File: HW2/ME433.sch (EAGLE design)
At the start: 22 parts, among them J1 USB-MB-H

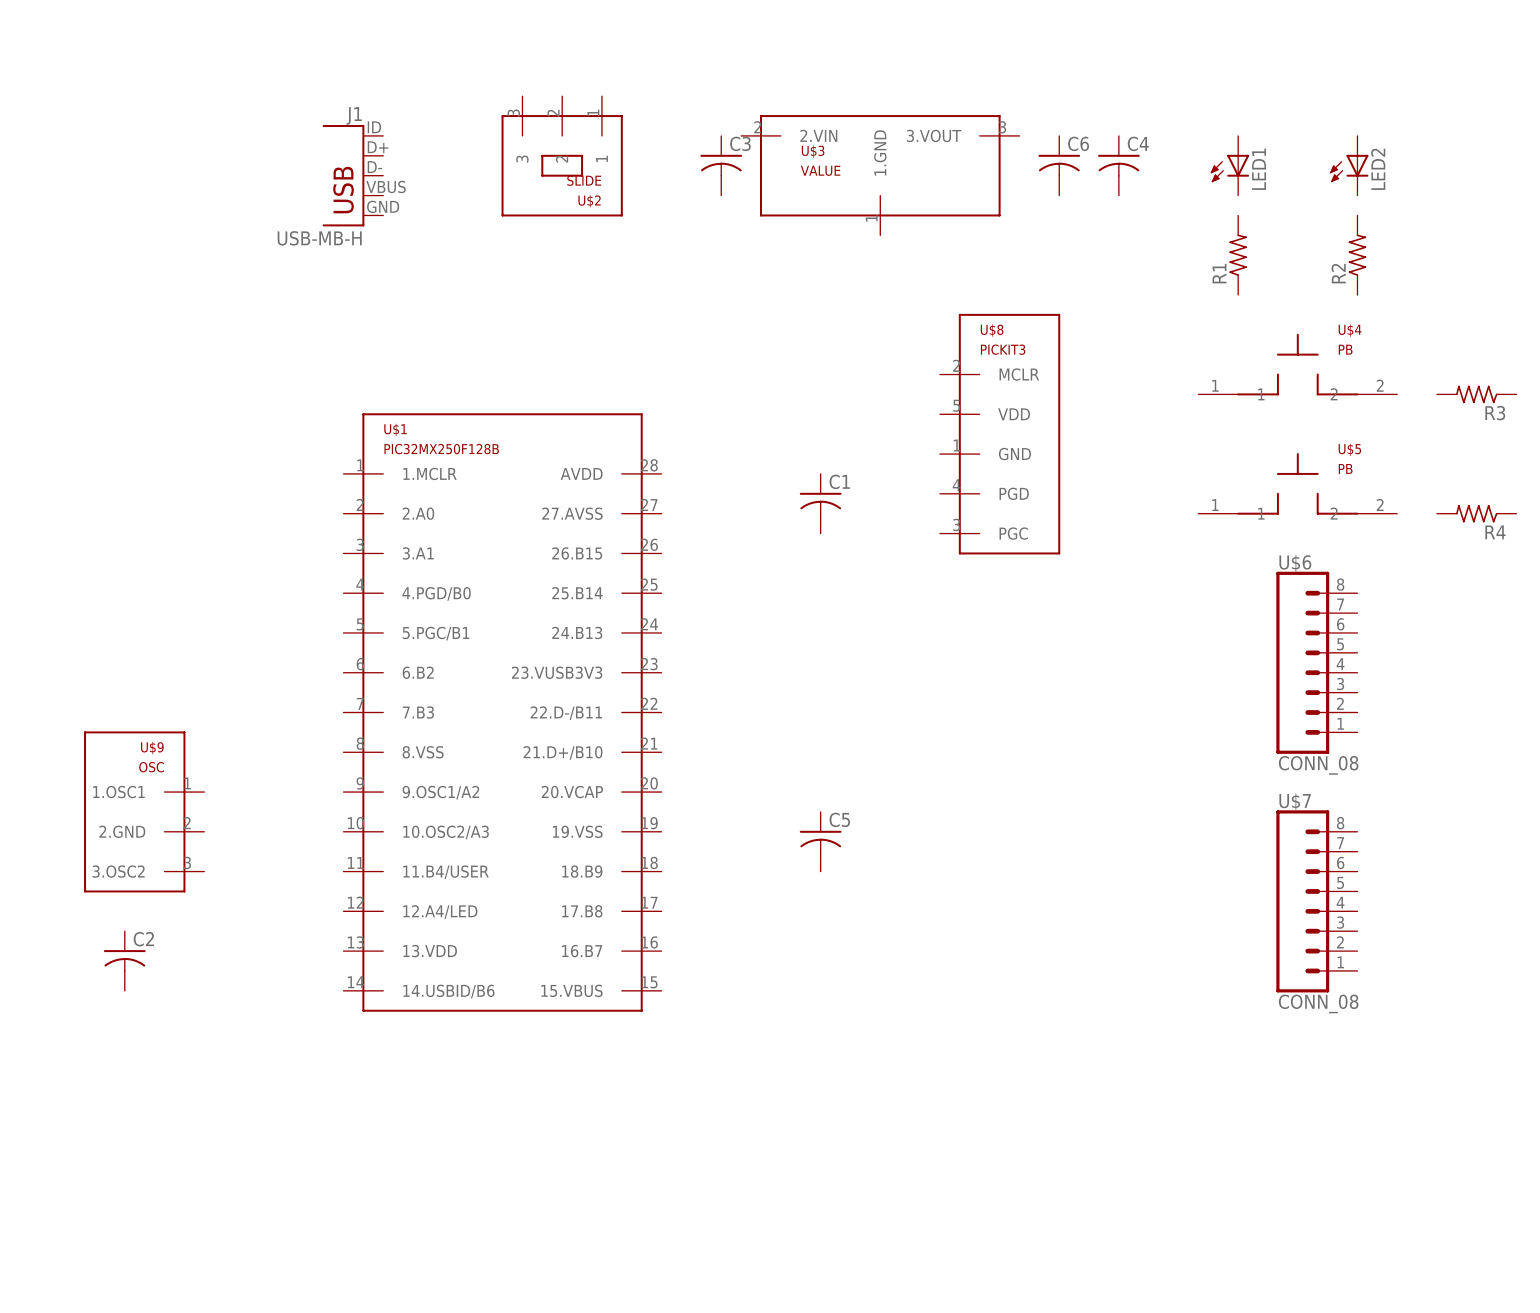
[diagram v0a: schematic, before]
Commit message: cleaned up HW2
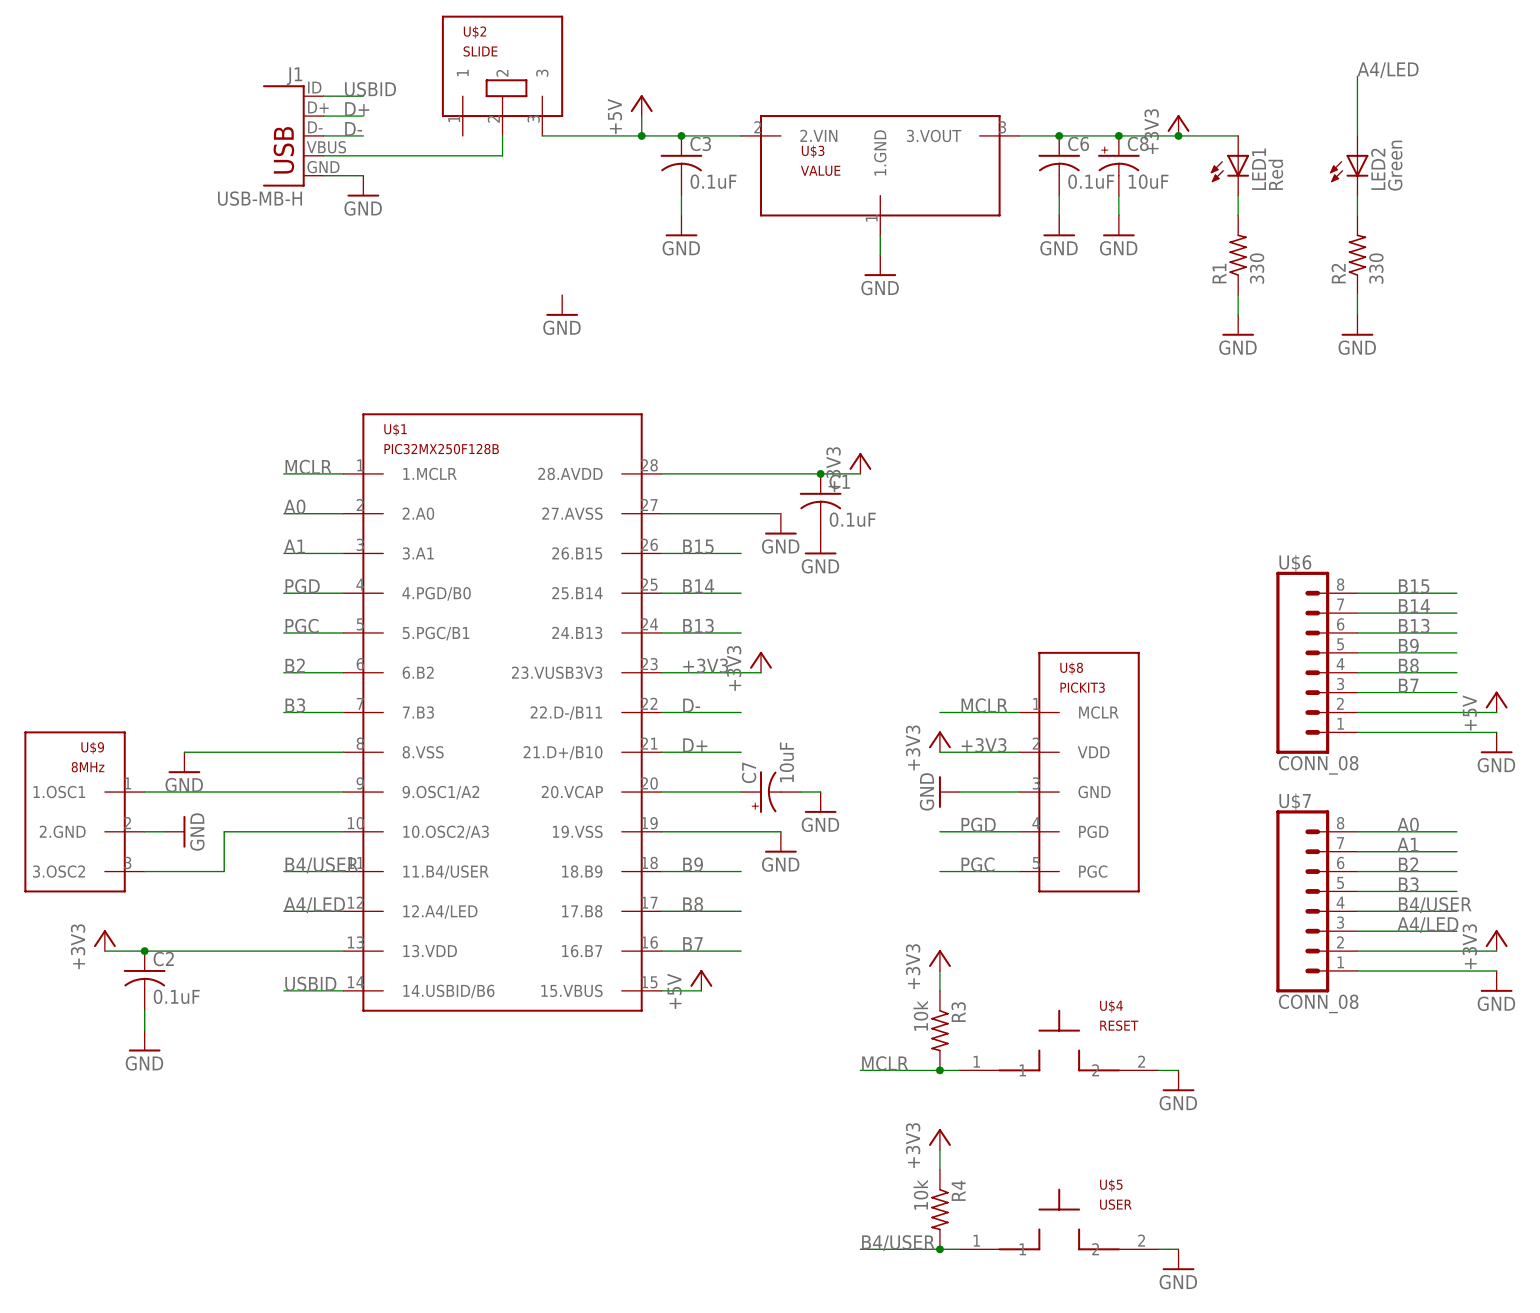
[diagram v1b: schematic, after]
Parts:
- removed C4, C5: (no value), resistor:C-US025-025X050
- added C7, C8: 10uF, HW2:CPOL-USB45181B
- C1, C2, C3, C6: value (none) -> 0.1uF
- LED1: value (none) -> Red
- LED2: value (none) -> Green
- R1, R2: value (none) -> 330
- R3, R4: value (none) -> 10k
- U$4: value PB -> RESET
- U$5: value PB -> USER
- U$9: value OSC -> 8MHz
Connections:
- new net +3V3: C1.1, C2.1, C6.1, C8.+, LED1.A, R3.1, R4.1, U$1.13.VDD, U$1.23.VUSB3V3, U$1.28.AVDD, U$3.3.VOUT, U$7.2, U$8.VDD
- new net +5V: C3.1, U$1.15.VBUS, U$2.3, U$3.2.VIN, U$6.2
- new net A0: U$1.2.A0, U$7.8
- new net A1: U$1.3.A1, U$7.7
- new net A4/LED: LED2.A, U$1.12.A4/LED, U$7.3
- new net B13: U$1.24.B13, U$6.6
- new net B14: U$1.25.B14, U$6.7
- new net B15: U$1.26.B15, U$6.8
- new net B2: U$1.6.B2, U$7.6
- new net B3: U$1.7.B3, U$7.5
- new net B4/USER: R4.2, U$1.11.B4/USER, U$5.1, U$7.4
- new net B7: U$1.16.B7, U$6.3
- new net B8: U$1.17.B8, U$6.4
- new net B9: U$1.18.B9, U$6.5
- new net D+: J1.D+, U$1.21.D+/B10
- new net D-: J1.D-, U$1.22.D-/B11
- new net GND: C1.2, C2.2, C3.2, C6.2, C7.-, C8.-, J1.GND, R1.1, R2.1, U$1.19.VSS, U$1.27.AVSS, U$1.8.VSS, U$3.1.GND, U$4.2, U$5.2, U$6.1, U$7.1, U$8.GND, U$9.2.GND
- new net MCLR: R3.2, U$1.1.MCLR, U$4.1, U$8.MCLR
- new net N$1: J1.VBUS, U$2.2
- new net N$2: U$1.9.OSC1/A2, U$9.1.OSC1
- new net N$3: U$1.10.OSC2/A3, U$9.3.OSC2
- new net N$4: LED1.C, R1.2
- new net N$5: C7.+, U$1.20.VCAP
- new net N$7: LED2.C, R2.2
- new net PGC: U$1.5.PGC/B1, U$8.PGC
- new net PGD: U$1.4.PGD/B0, U$8.PGD
- new net USBID: J1.D+1, U$1.14.USBID/B6
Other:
- moved on the sheet: C2, C3, J1, R3, R4, U$2, U$4, U$5, U$8, U$9
